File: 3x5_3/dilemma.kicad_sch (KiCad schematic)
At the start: 252 parts, among them J1 USB_C_Receptacle_USB2.0, J102 NA_serial, J105 NA_Conn_01x04_Female, J113 Cirque, J3 NA_GC9A01, J4 Conn_01x05, J5 NA_Conn_01x02, J5001 USB_C_Receptacle_USB2.0, J5002 NA_Conn_01x02, J5003 NA_serial, J5004 NA_GC9A01, J5005 NA_Conn_01x04_Female, J5007 Cirque, J5008 Conn_01x05, J5009 Conn_01x05, J5010 Conn_01x05, SW1 SW_Push, SW101 NA_SW_Push, SW102 NA_SW_Push, SW103 NA_SW_Push, SW104 NA_SW_Push, SW105 NA_SW_Push, SW106 NA_SW_Push, SW107 NA_SW_Push, SW108 NA_SW_Push, SW109 NA_SW_Push, SW112 NA_SW_Push, SW113 NA_SW_Push, SW114 NA_SW_Push, SW115 NA_SW_Push, SW116 NA_SW_Push, SW117 NA_SW_Push, SW118 NA_SW_Push, SW119 NA_SW_Push, SW3001 NA_SW_Push, SW3002 NA_RotaryEncoder_Switch, SW5001 SW_Push, SW5002 NA_SW_Push, SW5003 NA_SW_Push, SW5004 NA_SW_Push, SW5005 NA_SW_Push, SW5006 NA_SW_Push, SW5007 NA_SW_Push, SW5008 NA_SW_Push, SW5009 NA_SW_Push, SW5010 NA_SW_Push, SW5011 NA_SW_Push, SW5012 NA_SW_Push, SW5013 NA_SW_Push, SW5014 NA_SW_Push, SW5015 NA_SW_Push, SW5016 NA_SW_Push, SW5017 NA_SW_Push, SW5018 NA_SW_Push, SW5019 NA_SW_Push, SW5020 NA_RotaryEncoder_Switch, SW5021 SW_SPST, SW5022 SW_SPST, U1 RP2040, U2 W25Q128JVS, U3 XC6210B332MR-G, U4 USBLC6-2P6, U5001 XC6210B332MR-G, U5002 RP2040, U5003 USBLC6-2P6, U5004 W25Q128JVS, U5005 USBLC6-2P6, U5006 USBLC6-2P6, Y1 Crystal_GND24, Y5001 Crystal_GND24

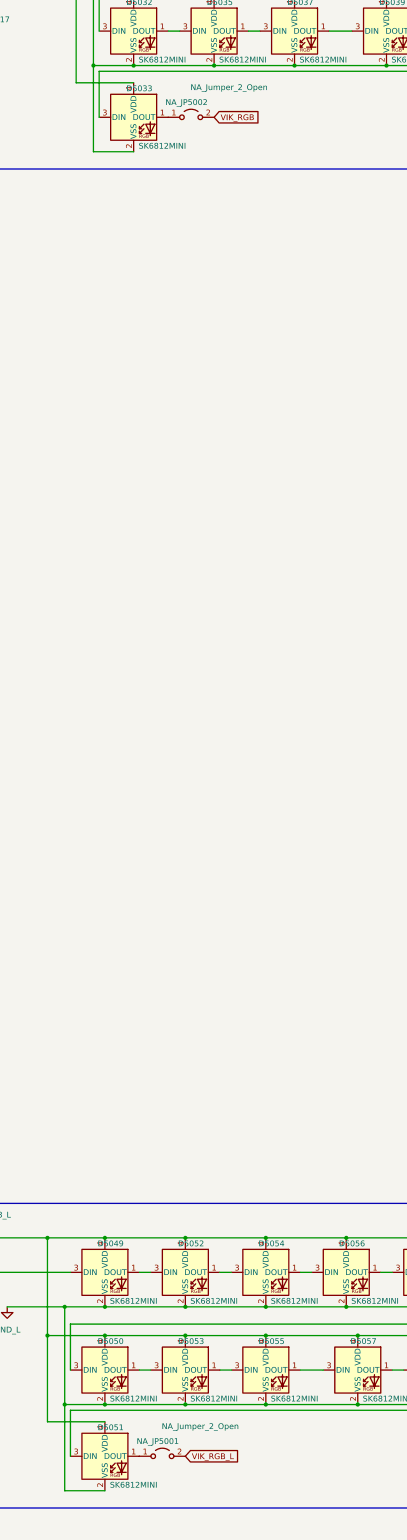
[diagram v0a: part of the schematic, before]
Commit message: DRC, leds
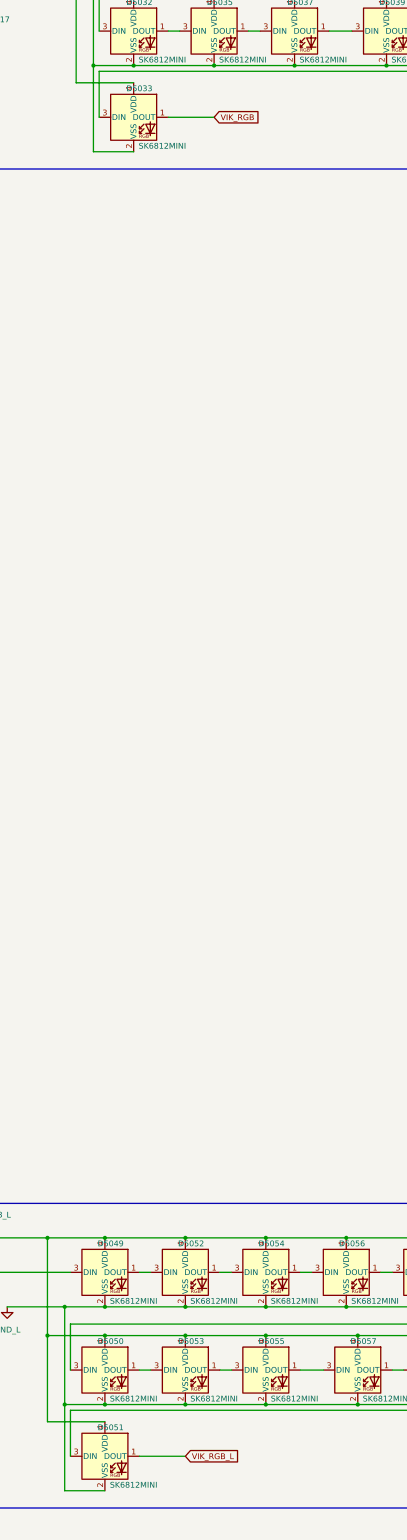
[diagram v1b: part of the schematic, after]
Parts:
- removed NA_JP5001, NA_JP5002: NA_Jumper_2_Open, local-libraries:SolderJumper-2_P1.3mm_Open_RoundedPad1.0x1.5mm, symbol Jumper:Jumper_2_Open
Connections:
- net VIK_RGB: now also D5033.1 (DOUT)
- net VIK_RGB_L: now also D5051.1 (DOUT)
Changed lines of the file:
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@@
 	(wire
 		(pts
+			(xy 628.65 76.2) (xy 638.81 76.2)
+		)
+		(stroke
+			(width 0)
+			(type default)
+		)
+	)
+	(wire
+		(pts
 			(xy 97.79 106.68) (xy 105.41 106.68)
 		)
@@
 	(wire
 		(pts
+			(xy 622.3 372.11) (xy 632.46 372.11)
+		)
+		(stroke
+			(width 0)
+			(type default)
+		)
+	)
+	(wire
+		(pts
 			(xy 455.93 359.41) (xy 473.71 359.41)
 		)
@@
 	)
 	(symbol
-		(lib_id "Jumper:Jumper_2_Open")
-		(at 633.73 76.2 0)
-		(unit 1)
-		(exclude_from_sim no)
-		(in_bom no)
-		(on_board yes)
-		(dnp no)
-		(property "Reference" "NA_JP5002"
-			(at 632.714 72.898 0)
-			(effects
-				(font
-					(size 1.27 1.27)
-				)
-			)
-		)
-		(property "Value" "NA_Jumper_2_Open"
-			(at 642.112 69.596 0)
-			(effects
-				(font
-					(size 1.27 1.27)
-				)
-			)
-		)
-		(property "Footprint" "local-libraries:SolderJumper-2_P1.3mm_Open_RoundedPad1.0x1.5mm"
-			(at 633.73 76.2 0)
-			(effects
-				(font
-					(size 1.27 1.27)
-				)
-				(hide yes)
-			)
-		)
-		(property "Datasheet" "~"
-			(at 633.73 76.2 0)
-			(effects
-				(font
-					(size 1.27 1.27)
-				)
-				(hide yes)
-			)
-		)
-		(property "Description" ""
-			(at 633.73 76.2 0)
-			(effects
-				(font
-					(size 1.27 1.27)
-				)
-				(hide yes)
-			)
-		)
-		(pin "1"
-		)
-		(pin "2"
-		)
-		(instances
-			(project "dilemma"
-				(path "/7353e96a-343a-4876-b497-b1d205a14d97"
-					(reference "NA_JP5002")
-					(unit 1)
-				)
-			)
-		)
-	)
-	(symbol
 		(lib_id "Switch:SW_Push")
 		(at 129.54 238.76 0)
@@
 					(unit 1)
 				)
-			)
-		)
-	)
-	(symbol
-		(lib_id "Jumper:Jumper_2_Open")
-		(at 627.38 372.11 0)
-		(unit 1)
-		(exclude_from_sim no)
-		(in_bom no)
-		(on_board yes)
-		(dnp no)
-		(property "Reference" "NA_JP5001"
-			(at 626.364 368.808 0)
-			(effects
-				(font
-					(size 1.27 1.27)
-				)
-			)
-		)
-		(property "Value" "NA_Jumper_2_Open"
-			(at 635.762 365.506 0)
-			(effects
-				(font
-					(size 1.27 1.27)
-				)
-			)
-		)
-		(property "Footprint" "local-libraries:SolderJumper-2_P1.3mm_Open_RoundedPad1.0x1.5mm"
-			(at 627.38 372.11 0)
-			(effects
-				(font
-					(size 1.27 1.27)
-				)
-				(hide yes)
-			)
-		)
-		(property "Datasheet" "~"
-			(at 627.38 372.11 0)
-			(effects
-				(font
-					(size 1.27 1.27)
-				)
-				(hide yes)
-			)
-		)
-		(property "Description" ""
-			(at 627.38 372.11 0)
-			(effects
-				(font
-					(size 1.27 1.27)
-				)
-				(hide yes)
-			)
-		)
-		(pin "1"
-		)
-		(pin "2"
-		)
-		(instances
-			(project "dilemma"
-				(path "/7353e96a-343a-4876-b497-b1d205a14d97"
-					(reference "NA_JP5001")
-					(unit 1)
-				)
